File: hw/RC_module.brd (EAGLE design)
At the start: 25 x 45 mm, 44 parts, among them J1 GROVE-4P-2.0-3470130P1, J2 GROVE-4P-2.0-3470130P1, X1 22-23-2021

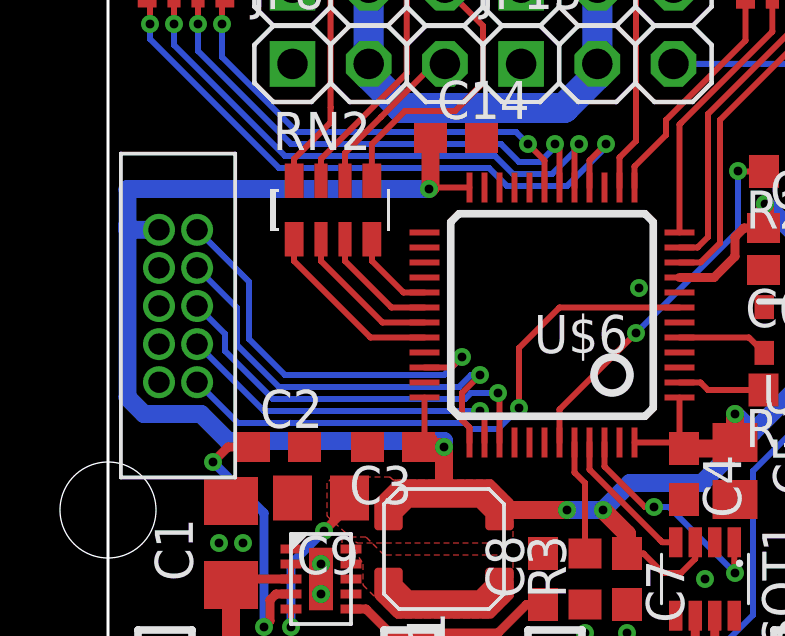
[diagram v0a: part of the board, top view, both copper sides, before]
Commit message: layout completed
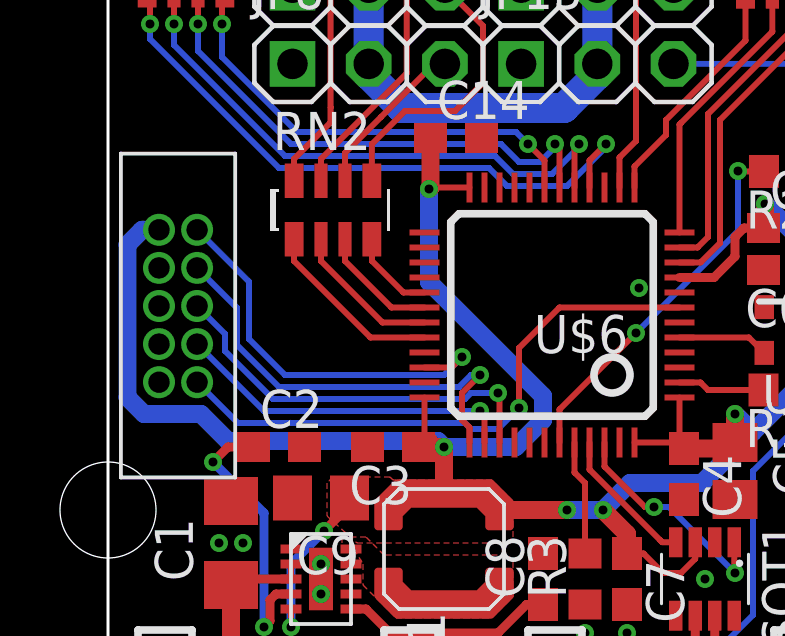
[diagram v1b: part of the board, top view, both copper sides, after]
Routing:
- net +3V3: track 84.3 -> 85.3 mm
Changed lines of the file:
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@@
 <wire x1="1.2" y1="13.2" x2="3.1" y2="13.2" width="0.6" layer="16"/>
 <wire x1="3.1" y1="13.2" x2="4" y2="12.3" width="0.6" layer="16"/>
-<wire x1="4" y1="12.3" x2="11.2" y2="12.3" width="0.6" layer="16"/>
-<wire x1="11.2" y1="12.3" x2="11.2" y2="12.1" width="0.6" layer="16"/>
 <wire x1="7.2" y1="9.3" x2="8.05" y2="10.15" width="0.3" layer="1"/>
 <wire x1="8.05" y1="10.15" x2="8.05" y2="10.4" width="0.3" layer="1"/>
@@
 <wire x1="21.85" y1="19.4" x2="21.9" y2="19.45" width="0.6" layer="1"/>
 <wire x1="21.9" y1="19.45" x2="21.9" y2="20.2" width="0.6" layer="1"/>
-<wire x1="0.65" y1="13.75" x2="0.65" y2="19.5" width="0.6" layer="16"/>
-<wire x1="0.65" y1="19.5" x2="0.65" y2="20.7" width="0.6" layer="16"/>
-<wire x1="0.65" y1="20.7" x2="10.7" y2="20.7" width="0.6" layer="16"/>
-<wire x1="1.7" y1="19.34" x2="0.65" y2="19.34" width="0.6" layer="16"/>
-<wire x1="0.65" y1="19.34" x2="0.65" y2="19.5" width="0.6" layer="16"/>
 <contactref element="U$5" pad="4"/>
 <contactref element="U$5" pad="1"/>
@@
 <wire x1="21.9" y1="20.2" x2="24.3" y2="17.8" width="0.6" layer="16"/>
 <wire x1="24.3" y1="17.8" x2="24.3" y2="16" width="0.6" layer="16"/>
+<wire x1="0.65" y1="13.75" x2="0.65" y2="18.85" width="0.6" layer="16"/>
+<wire x1="0.65" y1="18.85" x2="1.1" y2="19.3" width="0.6" layer="16"/>
+<wire x1="1.7" y1="19.34" x2="1.14" y2="19.34" width="0.6" layer="16"/>
+<wire x1="1.14" y1="19.34" x2="1.1" y2="19.3" width="0.6" layer="16"/>
+<wire x1="10.7" y1="20.7" x2="10.7" y2="17.6" width="0.6" layer="16"/>
+<wire x1="10.7" y1="17.6" x2="14.5" y2="13.8" width="0.6" layer="16"/>
+<wire x1="4" y1="12.3" x2="11" y2="12.3" width="0.6" layer="16"/>
+<wire x1="11" y1="12.3" x2="11.2" y2="12.1" width="0.6" layer="16"/>
+<wire x1="13.6" y1="12.1" x2="11.2" y2="12.1" width="0.6" layer="16"/>
+<wire x1="14.5" y1="13.8" x2="14.5" y2="13" width="0.6" layer="16"/>
+<wire x1="14.5" y1="13" x2="13.6" y2="12.1" width="0.6" layer="16"/>
 </signal>
 <signal name="JTMS">

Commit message: added R values
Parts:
- R2: value 10k -> 330
- RN1: value (none) -> 330
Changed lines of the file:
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@@
 <element name="JP12" library="connectors" package="1X03" value="PINHD-3" x="16.31" y="27.41"/>
 <element name="JP13" library="connectors" package="1X03" value="PINHD-3" x="16.31" y="24.87"/>
-<element name="RN1" library="dp_devices" package="RN8P-4R-CRA06S" value="" x="2.6" y="28.3"/>
+<element name="RN1" library="dp_devices" package="RN8P-4R-CRA06S" value="330" x="2.6" y="28.3"/>
 <element name="RN2" library="dp_devices" package="RN8P-4R-CRA06S" value="" x="7.5" y="20"/>
 <element name="RN3" library="dp_devices" package="RN8P-4R-CRA06S" value="" x="22.545" y="28.26"/>
@@
 <element name="JP7" library="connectors" package="1X03" value="PINHD-3" x="8.69" y="27.41"/>
 <element name="JP8" library="connectors" package="1X03" value="PINHD-3" x="8.69" y="24.87"/>
-<element name="R2" library="rcl" package="R0603" value="10k" x="22.715" y="21.285" rot="R180"/>
+<element name="R2" library="rcl" package="R0603" value="330" x="22.715" y="21.285" rot="R180"/>
 <element name="R4" library="rcl" package="R0603" value="10k" x="21.5" y="42.5" rot="R180"/>
 <element name="R5" library="rcl" package="R0603" value="10k" x="21.5" y="41.1"/>

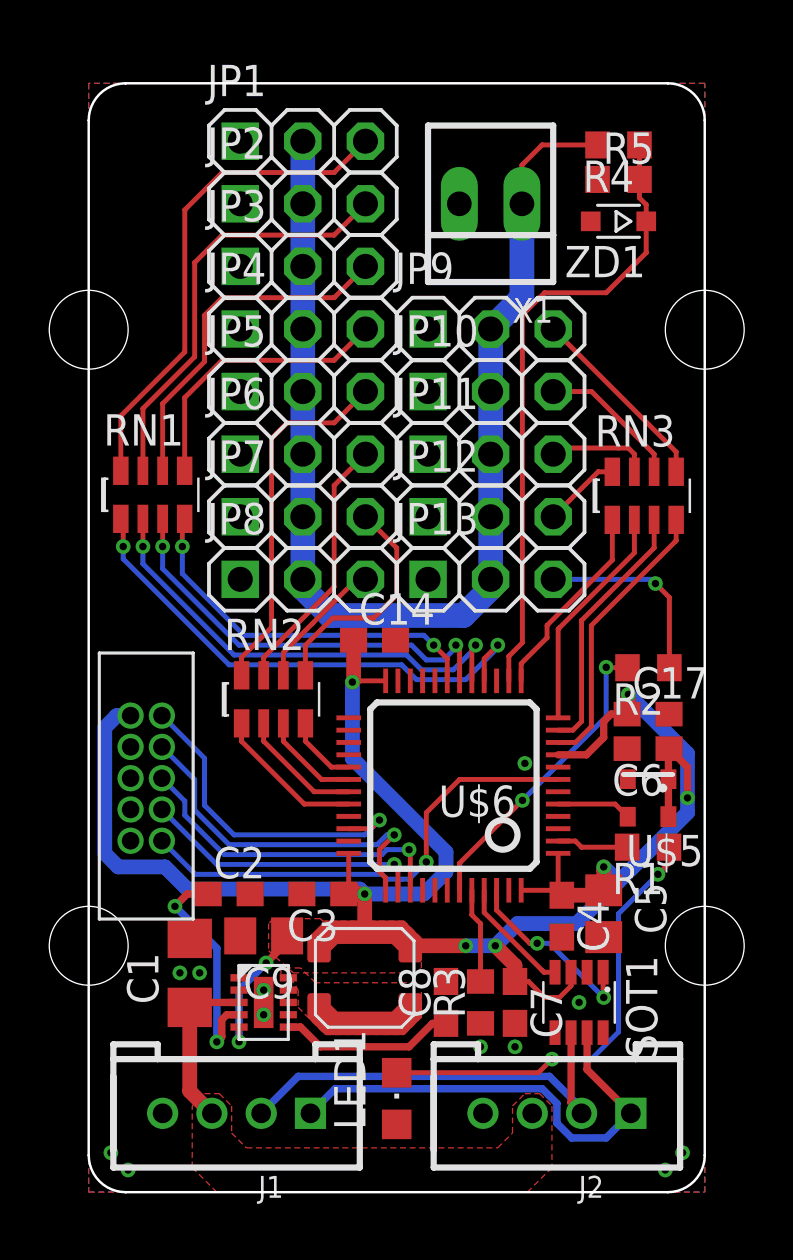
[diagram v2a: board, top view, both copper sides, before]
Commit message: small fixes
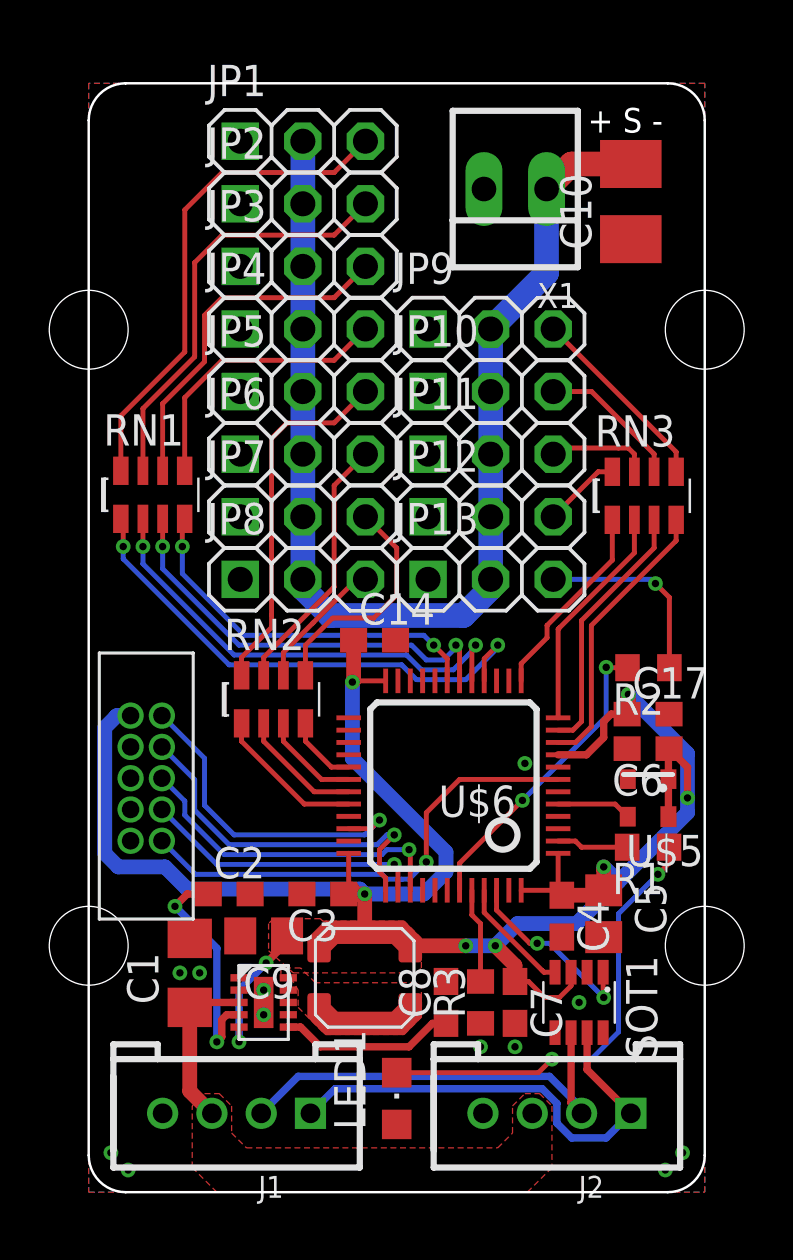
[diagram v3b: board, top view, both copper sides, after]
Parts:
- removed R4, R5: 10k, rcl:R0603
- removed ZD1: (no value), dp_devices:SOD-323F
- added C10: (no value), rcl:B/3528-21R
- moved X1 1.17 mm to (17.3, 40.7)
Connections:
- net +V: now also C10.+; no longer R4.2
- net GND: now also C10.-; no longer R5.1, ZD1.A
- net VSENSE: no longer R4.1, R5.2, ZD1.C
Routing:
- net VSENSE: track 25.6 -> 0.00 mm
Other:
- board text added: "+ S -"
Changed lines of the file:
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@@
 <?xml version="1.0" encoding="utf-8"?>
 <!DOCTYPE eagle SYSTEM "eagle.dtd">
-<eagle version="6.4">
+<eagle version="7.2.0">
 <drawing>
 <settings>
@@
 <layers>
 <layer number="1" name="Top" color="4" fill="1" visible="yes" active="yes"/>
-<layer number="16" name="Bottom" color="1" fill="1" visible="no" active="yes"/>
+<layer number="16" name="Bottom" color="1" fill="1" visible="yes" active="yes"/>
 <layer number="17" name="Pads" color="2" fill="1" visible="yes" active="yes"/>
 <layer number="18" name="Vias" color="2" fill="1" visible="yes" active="yes"/>
@@
 <layer number="46" name="Milling" color="3" fill="1" visible="yes" active="yes"/>
 <layer number="47" name="Measures" color="7" fill="1" visible="no" active="yes"/>
-<layer number="48" name="Document" color="7" fill="1" visible="no" active="yes"/>
+<layer number="48" name="Document" color="7" fill="1" visible="yes" active="yes"/>
 <layer number="49" name="Reference" color="7" fill="1" visible="no" active="yes"/>
 <layer number="50" name="dxf" color="7" fill="1" visible="no" active="no"/>
@@
 <wire x1="6.55" y1="8" x2="6.55" y2="8.8" width="0.2" layer="41"/>
 <wire x1="6.55" y1="8.8" x2="7.45" y2="8.8" width="0.2" layer="41"/>
+<text x="23.3" y="44" size="1" layer="20" rot="R180">+ S -</text>
 </plain>
 <attributes>
@@
 <pass name="Default">
 <param name="RoutingGrid" value="50mil"/>
+<param name="AutoGrid" value="1"/>
+<param name="Efforts" value="0"/>
+<param name="TopRouterVariant" value="1"/>
 <param name="tpViaShape" value="round"/>
 <param name="PrefDir.1" value="|"/>
@@
 <element name="RN2" library="dp_devices" package="RN8P-4R-CRA06S" value="" x="7.5" y="20"/>
 <element name="RN3" library="dp_devices" package="RN8P-4R-CRA06S" value="" x="22.545" y="28.26"/>
-<element name="X1" library="con-molex" package="22-23-2021" value="22-23-2021" x="16.31" y="40.11" rot="R180">
-<attribute name="OC_NEWARK" value="25C3832" x="16.31" y="40.11" size="1.778" layer="27" rot="R180" display="off"/>
-<attribute name="MPN" value="22-23-2021" x="16.31" y="40.11" size="1.778" layer="27" rot="R180" display="off"/>
-<attribute name="MF" value="MOLEX" x="16.31" y="40.11" size="1.778" layer="27" rot="R180" display="off"/>
-<attribute name="OC_FARNELL" value="1462926" x="16.31" y="40.11" size="1.778" layer="27" rot="R180" display="off"/>
+<element name="X1" library="con-molex" package="22-23-2021" value="22-23-2021" x="17.31" y="40.71" rot="R180">
+<attribute name="OC_NEWARK" value="25C3832" x="17.31" y="40.71" size="1.778" layer="27" rot="R180" display="off"/>
+<attribute name="MPN" value="22-23-2021" x="17.31" y="40.71" size="1.778" layer="27" rot="R180" display="off"/>
+<attribute name="MF" value="MOLEX" x="17.31" y="40.71" size="1.778" layer="27" rot="R180" display="off"/>
+<attribute name="OC_FARNELL" value="1462926" x="17.31" y="40.71" size="1.778" layer="27" rot="R180" display="off"/>
 </element>
 <element name="JP9" library="connectors" package="1X03" value="PINHD-3" x="16.31" y="35.03"/>
@@
 <element name="JP8" library="connectors" package="1X03" value="PINHD-3" x="8.69" y="24.87"/>
 <element name="R2" library="rcl" package="R0603" value="330" x="22.715" y="21.285" rot="R180"/>
-<element name="R4" library="rcl" package="R0603" value="10k" x="21.5" y="42.5" rot="R180"/>
-<element name="R5" library="rcl" package="R0603" value="10k" x="21.5" y="41.1"/>
-<element name="ZD1" library="dp_devices" package="SOD-323F" value="" x="21.5" y="39.4" rot="R180"/>
+<element name="C10" library="rcl" package="B/3528-21R" value="" x="22" y="40.2" rot="R90"/>
 </elements>
 <signals>
@@
 <contactref element="JP8" pad="1"/>
 <contactref element="JP7" pad="1"/>
-<contactref element="R5" pad="1"/>
-<contactref element="ZD1" pad="A"/>
+<contactref element="C10" pad="-"/>
 </signal>
 <signal name="VIN">
@@
 <contactref element="JP8" pad="2"/>
 <wire x1="8.69" y1="29.95" x2="8.69" y2="27.41" width="1" layer="16"/>
-<wire x1="16.31" y1="35.03" x2="17.58" y2="36.3" width="1" layer="16"/>
-<wire x1="17.58" y1="36.3" x2="17.58" y2="40.11" width="1" layer="16"/>
 <wire x1="16.31" y1="24.87" x2="16.31" y2="24.51" width="1" layer="16"/>
 <wire x1="16.31" y1="24.51" x2="15.2" y2="23.4" width="1" layer="16"/>
@@
 <wire x1="8.69" y1="24.87" x2="8.69" y2="24.51" width="1" layer="16"/>
 <wire x1="8.69" y1="24.51" x2="9.8" y2="23.4" width="1" layer="16"/>
-<contactref element="R4" pad="2"/>
-<wire x1="20.65" y1="42.5" x2="18.4" y2="42.5" width="0.2" layer="1"/>
-<wire x1="17.58" y1="40.11" x2="17.58" y2="41.68" width="0.2" layer="1"/>
-<wire x1="17.58" y1="41.68" x2="18.4" y2="42.5" width="0.2" layer="1"/>
+<contactref element="C10" pad="+"/>
+<wire x1="22" y1="41.725" x2="19.595" y2="41.725" width="1" layer="1"/>
+<wire x1="19.595" y1="41.725" x2="18.58" y2="40.71" width="1" layer="1"/>
+<wire x1="18.58" y1="40.71" x2="18.58" y2="37.3" width="1" layer="16"/>
+<wire x1="18.58" y1="37.3" x2="16.31" y2="35.03" width="1" layer="16"/>
 </signal>
 <signal name="N$11">
@@
 <signal name="VSENSE">
 <contactref element="U$6" pad="14"/>
-<contactref element="R4" pad="1"/>
-<contactref element="R5" pad="2"/>
-<contactref element="ZD1" pad="C"/>
-<wire x1="22.35" y1="42.5" x2="22.35" y2="41.1" width="0.2" layer="1"/>
-<wire x1="22.35" y1="41.1" x2="22.35" y2="40.35" width="0.2" layer="1"/>
-<wire x1="22.625" y1="39.4" x2="22.625" y2="40.075" width="0.2" layer="1"/>
-<wire x1="22.625" y1="40.075" x2="22.35" y2="40.35" width="0.2" layer="1"/>
-<wire x1="22.625" y1="39.4" x2="22.625" y2="38.125" width="0.2" layer="1"/>
-<wire x1="22.625" y1="38.125" x2="21" y2="36.5" width="0.2" layer="1"/>
-<wire x1="21" y1="36.5" x2="18.5" y2="36.5" width="0.2" layer="1"/>
-<wire x1="18.5" y1="36.5" x2="17.6" y2="35.6" width="0.2" layer="1"/>
-<wire x1="17.6" y1="35.6" x2="17.6" y2="22.3" width="0.2" layer="1"/>
-<wire x1="17.05" y1="20.75" x2="17.05" y2="21.75" width="0.2" layer="1"/>
-<wire x1="17.05" y1="21.75" x2="17.6" y2="22.3" width="0.2" layer="1"/>
 </signal>
 </signals>
